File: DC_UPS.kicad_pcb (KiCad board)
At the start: 2 copper layers, 30.6 x 29.4 mm, 31 parts, among them Q1 SIS402DN, Q2 SIS402DN, U1 LTC4040

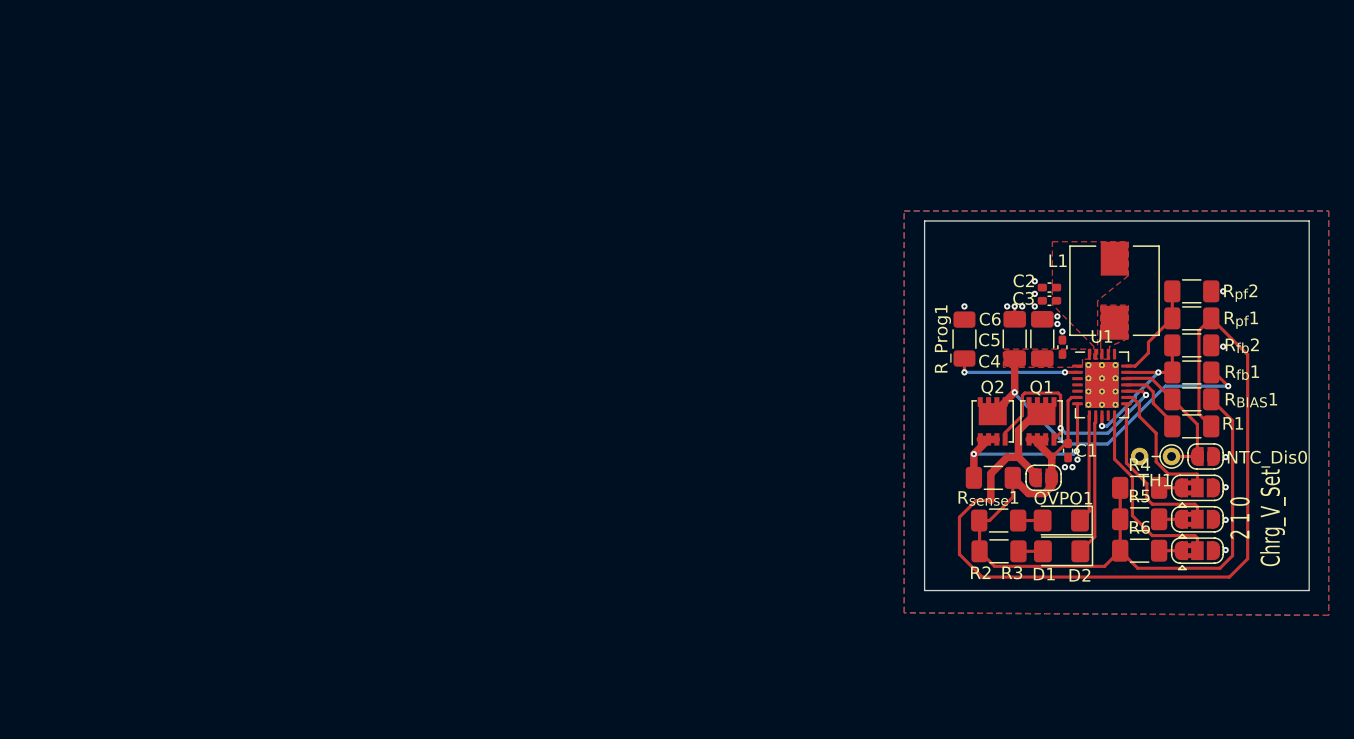
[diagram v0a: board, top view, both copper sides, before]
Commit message: [Board]Finish product rev 1
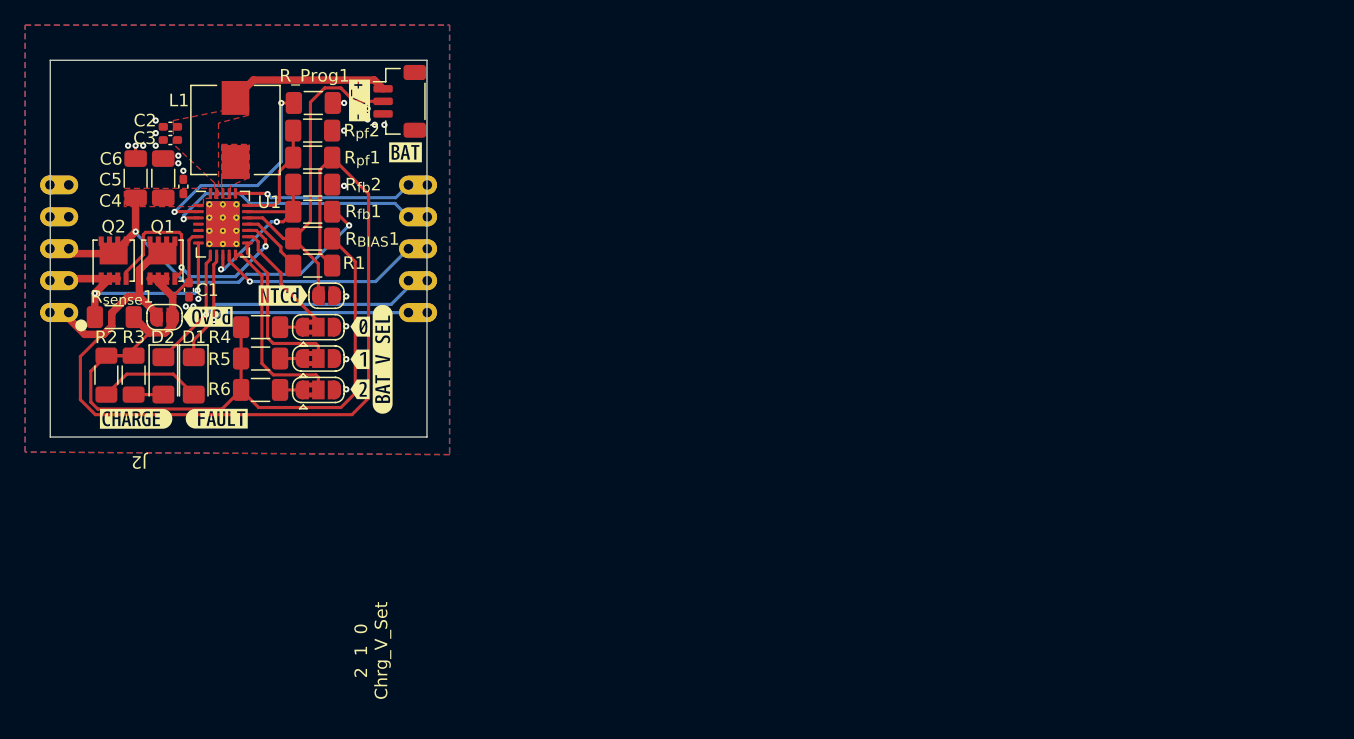
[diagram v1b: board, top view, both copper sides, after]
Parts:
- removed TH1: NTC, Resistor_THT:R_Axial_DIN0204_L3.6mm_D1.6mm_P2.54mm_Vertical
- added J2: POWER, Castellated_Header:CastellatedPinHeader_2.54mm_5, F.Cu at (31.5, 50.1)
- added J3: STATUS, Castellated_Header:CastellatedPinHeader_2.54mm_5, B.Cu at (58.5, 50.1)
- added J4: BAT_CONN, Connector_JST:JST_SH_BM03B-SRSS-TB_1x03-1MP_P1.00mm_Vertical, F.Cu at (57.8, 33.3)
- added kibuzzard-63A19CFD: G***, kibuzzard-63A19CFD, F.Cu at (54.7, 51.2)
- added kibuzzard-63A19D17: G***, kibuzzard-63A19D17, F.Cu at (54.7, 53.8)
- added kibuzzard-63A19D4B: G***, kibuzzard-63A19D4B, F.Cu at (54.7, 56.2)
- added kibuzzard-63A19E71: G***, kibuzzard-63A19E71, F.Cu at (56.5, 53.8)
- added kibuzzard-63A19F8A: G***, kibuzzard-63A19F8A, F.Cu at (42.5, 50.4)
- added kibuzzard-63A19F98: G***, kibuzzard-63A19F98, F.Cu at (48.5, 48.7)
- added kibuzzard-63A1A047: G***, kibuzzard-63A1A047, F.Cu at (58.3, 37.3)
- added kibuzzard-63A1A128: G***, kibuzzard-63A1A128, F.Cu at (54.6, 33.2)
- added kibuzzard-63A1A287: G***, kibuzzard-63A1A287, F.Cu at (43.3, 58.5)
- added kibuzzard-63A1A2AA: G***, kibuzzard-63A1A2AA, F.Cu at (36.8, 58.5)
- added kibuzzard-63A1A4C9: G***, kibuzzard-63A1A4C9, B.Cu at (35.7, 50.1)
- added kibuzzard-63A1A50F: G***, kibuzzard-63A1A50F, B.Cu at (35.0, 47.5)
- added kibuzzard-63A1A543: G***, kibuzzard-63A1A543, B.Cu at (35.3, 45.0)
- added kibuzzard-63A1A568: G***, kibuzzard-63A1A568, B.Cu at (34.2, 40.0)
- added kibuzzard-63A1A568: G***, kibuzzard-63A1A568, B.Cu at (34.2, 42.5)
- added kibuzzard-63A1A71E: G***, kibuzzard-63A1A71E, B.Cu at (54.3, 42.5)
- added kibuzzard-63A1A72A: G***, kibuzzard-63A1A72A, B.Cu at (53.5, 45.0)
- added kibuzzard-63A1A734: G***, kibuzzard-63A1A734, B.Cu at (54.7, 47.5)
- added kibuzzard-63A1A785: G***, kibuzzard-63A1A785, B.Cu at (55.1, 50.1)
- added kibuzzard-63A1A798: G***, kibuzzard-63A1A798, B.Cu at (53.1, 39.9)
- moved R2 72.5 mm to (34.5, 55.1), turned to -90 degrees
- moved D2 72.4 mm to (39.0, 55.1), turned to -90 degrees
- moved C1 71.2 mm to (41.0, 48.3)
- moved C2 71.2 mm to (39.6, 35.3)
- moved C3 71.2 mm to (39.6, 36.4)
- moved C4 71.2 mm to (40.6, 40.0)
- moved C5 71.2 mm to (39.0, 39.4)
- moved C6 71.2 mm to (36.8, 39.4)
- moved F_SEL0 71.2 mm to (51.4, 51.2)
- moved F_SEL1 71.2 mm to (51.4, 53.8)
- moved F_SEL2 71.2 mm to (51.4, 56.2)
- moved L1 71.2 mm to (44.8, 35.5)
- moved NTC_Dis0 71.2 mm to (52.0, 48.8)
- moved OVPO1 71.2 mm to (39.1, 50.5)
- moved Q1 71.2 mm to (38.9, 46.0)
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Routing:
- net /CLPROG: track 0.00 -> 20.9 mm, vias 0 -> 1
- net /~{CHRG}: track 8.66 -> 27.2 mm, vias 0 -> 1
- net /~{RST_OUT}: track 0.00 -> 16.5 mm, vias 0 -> 1
- net /NTC: track 11.8 -> 27.8 mm
- net /~{POWER_FAIL}: track 0.00 -> 14.3 mm, vias 0 -> 1
- net /~{FAULT}: track 11.3 -> 24.6 mm, vias 0 -> 1
- net /BAT_+: track 0.00 -> 12.6 mm
- net /CHRG_PROG: track 10.0 -> 17.7 mm
- net Net-(D1-Pad2): track 1.95 -> 8.31 mm
- net /Vin: track 62.9 -> 66.7 mm
- net /V_SYS: track 27.6 -> 31.3 mm
- net /Input_V: track 71.6 -> 75.0 mm
- net /CLN: track 16.9 -> 19.6 mm
- net /BSTFB: track 13.0 -> 14.7 mm
- net /F0: track 11.1 -> 9.82 mm
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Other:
- board size 30.6 x 29.4 mm -> 30 x 30 mm
